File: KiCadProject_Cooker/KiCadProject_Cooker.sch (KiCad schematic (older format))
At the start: 10 parts, among them U1 ESP32-WROOM

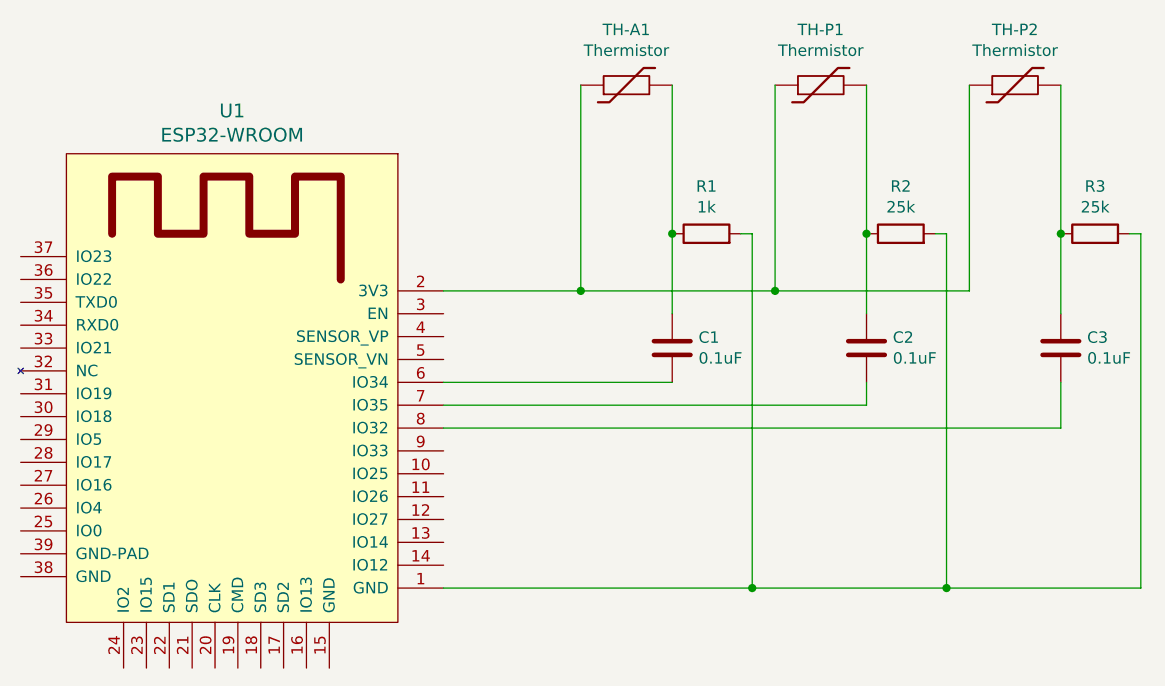
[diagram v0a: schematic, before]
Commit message: working and functional
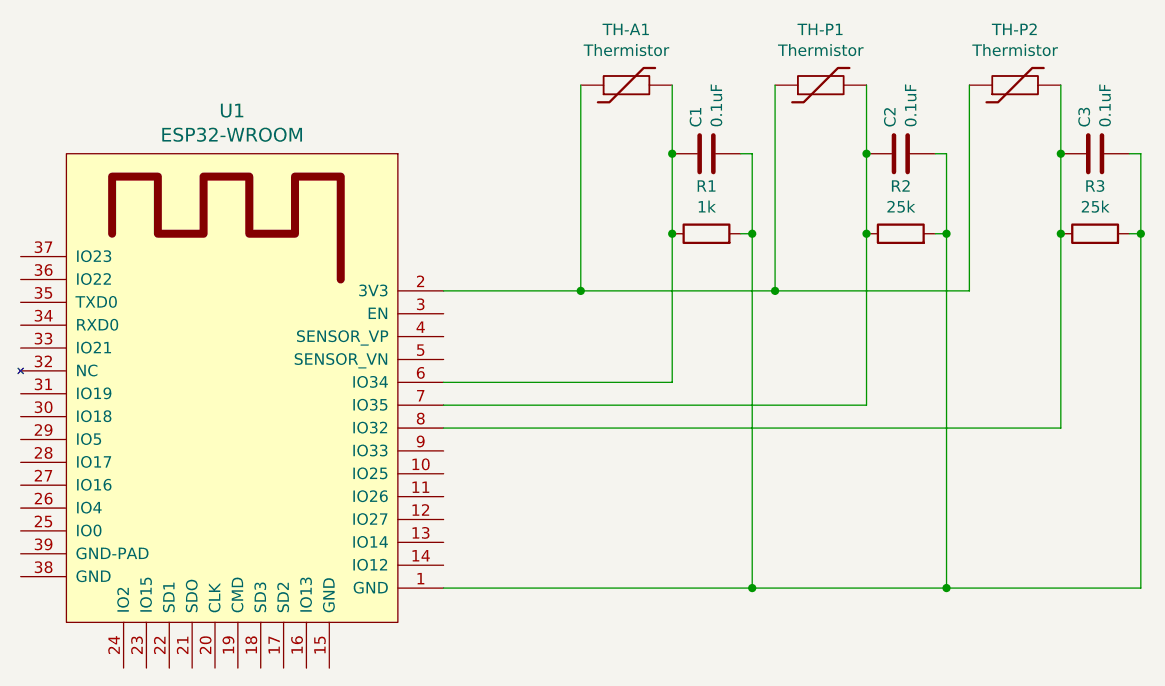
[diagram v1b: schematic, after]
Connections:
- net at C1.1, R1.1, TH-A1.2: now also U1.6 (IO34)
- net at R1.2, R2.2, R3.2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: now also C1.2, C2.2, C3.2
- net at C2.1, R2.1, TH-P1.2: now also U1.7 (IO35)
- net at C3.1, R3.1, TH-P2.2: now also U1.8 (IO32)
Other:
- moved on the sheet: C2, C3
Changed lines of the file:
@@
 $EndComp
 Wire Wire Line
-	4150 2050 4150 2700
+	4150 2050 4150 2350
 $Comp
 L Device:Thermistor TH-P1
@@
 $EndComp
 Wire Wire Line
-	5000 2050 5000 2700
+	5000 2050 5000 2350
 $Comp
 L Device:C C3
 U 1 1 6079633B
-P 5850 3200
-F 0 "C3" H 5965 3246 50  0000 L CNN
-F 1 "0.1uF" H 5965 3155 50  0000 L CNN
-F 2 "Capacitor_THT:C_Disc_D3.0mm_W1.6mm_P2.50mm" H 5888 3050 50  0001 C CNN
-F 3 "~" H 5850 3200 50  0001 C CNN
-	1    5850 3200
-	1    0    0    -1
+P 6000 2350
+F 0 "C3" H 6115 2396 50  0000 L CNN
+F 1 "0.1uF" H 6115 2305 50  0000 L CNN
+F 2 "Capacitor_THT:C_Disc_D3.0mm_W1.6mm_P2.50mm" H 6038 2200 50  0001 C CNN
+F 3 "~" H 6000 2350 50  0001 C CNN
+	1    6000 2350
+	0    -1   -1   0
 $EndComp
 $Comp
@@
 $EndComp
 Wire Wire Line
-	5850 2050 5850 2700
+	5850 2050 5850 2350
 Connection ~ 5850 2700
-Wire Wire Line
-	5850 2700 5850 3050
-Wire Wire Line
-	5000 3050 5000 2700
 Connection ~ 5000 2700
 $Comp
 L Device:C C2
 U 1 1 6079F8A7
-P 5000 3200
-F 0 "C2" H 5115 3246 50  0000 L CNN
-F 1 "0.1uF" H 5115 3155 50  0000 L CNN
-F 2 "Capacitor_THT:C_Disc_D3.0mm_W1.6mm_P2.50mm" H 5038 3050 50  0001 C CNN
-F 3 "~" H 5000 3200 50  0001 C CNN
-	1    5000 3200
-	1    0    0    -1
+P 5150 2350
+F 0 "C2" H 5265 2396 50  0000 L CNN
+F 1 "0.1uF" H 5265 2305 50  0000 L CNN
+F 2 "Capacitor_THT:C_Disc_D3.0mm_W1.6mm_P2.50mm" H 5188 2200 50  0001 C CNN
+F 3 "~" H 5150 2350 50  0001 C CNN
+	1    5150 2350
+	0    -1   -1   0
 $EndComp
-$Comp
-L Device:C C1
-U 1 1 607A05E2
-P 4150 3200
-F 0 "C1" H 4265 3246 50  0000 L CNN
-F 1 "0.1uF" H 4265 3155 50  0000 L CNN
-F 2 "Capacitor_THT:C_Disc_D3.0mm_W1.6mm_P2.50mm" H 4188 3050 50  0001 C CNN
-F 3 "~" H 4150 3200 50  0001 C CNN
-	1    4150 3200
-	1    0    0    -1
-$EndComp
-Wire Wire Line
-	4150 3050 4150 2700
 Connection ~ 4150 2700
 Wire Wire Line
@@
 	4150 3350 3150 3350
 Wire Wire Line
-	5000 3350 5000 3450
-Wire Wire Line
 	5000 3450 3150 3450
-Wire Wire Line
-	5850 3350 5850 3550
 Wire Wire Line
 	5850 3550 3150 3550
@@
 	-1   0    0    -1
 $EndComp
+$Comp
+L Device:C C1
+U 1 1 60817F0F
+P 4300 2350
+F 0 "C1" H 4415 2396 50  0000 L CNN
+F 1 "0.1uF" H 4415 2305 50  0000 L CNN
+F 2 "Capacitor_THT:C_Disc_D3.0mm_W1.6mm_P2.50mm" H 4338 2200 50  0001 C CNN
+F 3 "~" H 4300 2350 50  0001 C CNN
+	1    4300 2350
+	0    -1   -1   0
+$EndComp
+Wire Wire Line
+	4150 2700 4150 3350
+Wire Wire Line
+	5000 2700 5000 3450
+Wire Wire Line
+	5850 2700 5850 3550
+Connection ~ 4150 2350
+Wire Wire Line
+	4150 2350 4150 2700
+Connection ~ 5000 2350
+Wire Wire Line
+	5000 2350 5000 2700
+Connection ~ 5850 2350
+Wire Wire Line
+	5850 2350 5850 2700
+Wire Wire Line
+	4450 2350 4500 2350
+Wire Wire Line
+	4500 2350 4500 2700
+Connection ~ 4500 2700
+Wire Wire Line
+	5300 2350 5350 2350
+Wire Wire Line
+	5350 2350 5350 2700
+Connection ~ 5350 2700
+Wire Wire Line
+	6150 2350 6200 2350
+Wire Wire Line
+	6200 2350 6200 2700
+Connection ~ 6200 2700
 $EndSCHEMATC
